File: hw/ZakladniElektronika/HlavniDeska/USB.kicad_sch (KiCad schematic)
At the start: 18 parts, among them J2 USB_C_Receptacle_USB2.0, U13 TPD4E02B04DQA, U4 AP33772

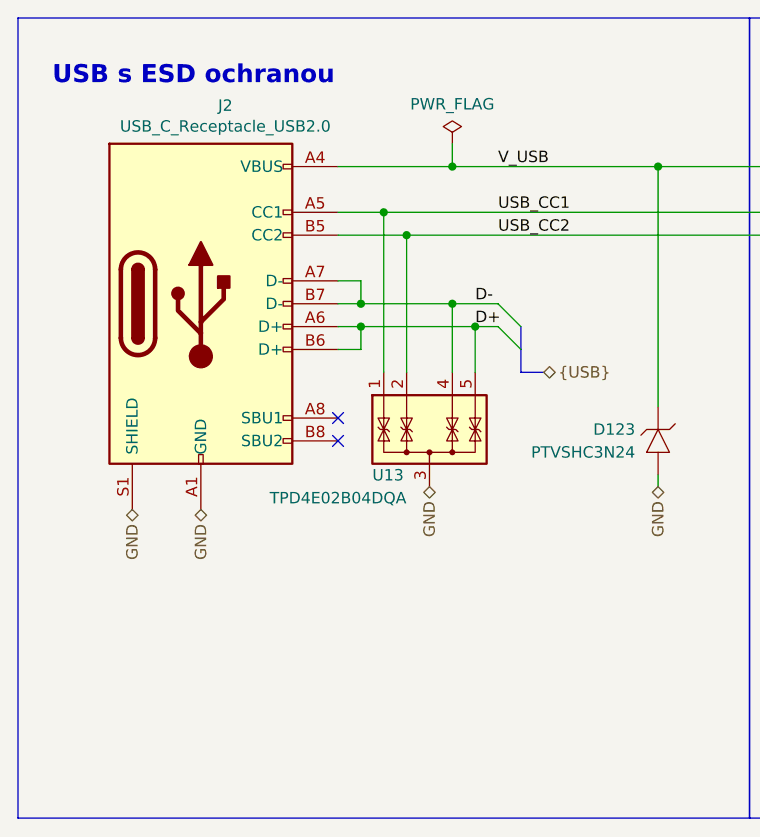
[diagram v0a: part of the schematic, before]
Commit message: WIP
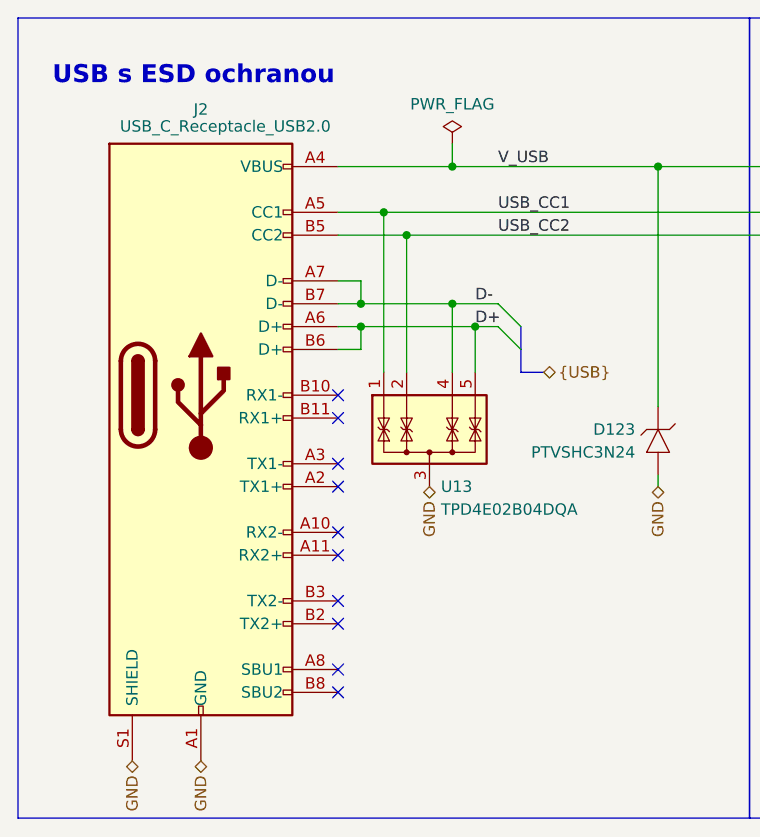
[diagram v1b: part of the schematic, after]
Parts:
- J2: symbol Connector:USB_C_Receptacle_USB2.0 -> Connector:USB_C_Receptacle
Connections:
- no-connect marks 7 -> 15
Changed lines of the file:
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@@
   )
   (no_connect (at 220.98 100.33))
+  (no_connect (at 86.36 107.95))
   (no_connect (at 220.98 110.49))
+  (no_connect (at 86.36 123.19))
+  (no_connect (at 86.36 100.33))
+  (no_connect (at 86.36 115.57))
+  (no_connect (at 86.36 125.73))
+  (no_connect (at 86.36 102.87))
   (no_connect (at 86.36 95.25))
-  (no_connect (at 86.36 97.79))
+  (no_connect (at 86.36 92.71))
+  (no_connect (at 86.36 110.49))
+  (no_connect (at 86.36 118.11))
   (no_connect (at 220.98 81.28))
   (no_connect (at 220.98 90.17))
@@
     (effects (font (size 1.27 1.27)) (justify right))
   )
-  (hierarchical_label "GND" (shape bidirectional) (at 71.12 105.41 270) (fields_autoplaced)
-    (effects (font (size 1.27 1.27)) (justify right))
-  )
-  (hierarchical_label "GND" (shape bidirectional) (at 63.5 105.41 270) (fields_autoplaced)
+  (hierarchical_label "GND" (shape bidirectional) (at 71.12 133.35 270) (fields_autoplaced)
+    (effects (font (size 1.27 1.27)) (justify right))
+  )
+  (hierarchical_label "GND" (shape bidirectional) (at 63.5 133.35 270) (fields_autoplaced)
     (effects (font (size 1.27 1.27)) (justify right))
   )
@@
     )
   )
-  (symbol (lib_id "Connector:USB_C_Receptacle_USB2.0") (at 71.12 82.55 0) (unit 1)
-    (in_bom yes) (on_board yes) (dnp no)
-    (property "Reference" "J2" (at 73.8378 60.5282 0)
+  (symbol (lib_id "Connector:USB_C_Receptacle") (at 71.12 92.71 0) (unit 1)
+    (in_bom yes) (on_board yes) (dnp no)
+    (property "Reference" "J2" (at 71.12 60.96 0)
       (effects (font (size 1.27 1.27)))
     )
@@
       (effects (font (size 1.27 1.27)))
     )
-    (property "Footprint" "RKL-Connectors:USB31-TYPEC-33141-2FS" (at 74.93 82.55 0)
-      (effects (font (size 1.27 1.27)) hide)
-    )
-    (property "Datasheet" "https://www.usb.org/sites/default/files/documents/usb_type-c.zip" (at 74.93 82.55 0)
-      (effects (font (size 1.27 1.27)) hide)
-    )
-    (property "LCSC" "C480368" (at 71.12 82.55 0)
-      (effects (font (size 1.27 1.27)) hide)
-    )
-    (property "JLCPCB_CORRECTION" "0;-1;0" (at 71.12 82.55 0)
-      (effects (font (size 1.27 1.27)) hide)
-    )
-    (property "Basic/Extended" "E" (at 71.12 82.55 0)
+    (property "Footprint" "RKL-Connectors:USB31-TYPEC-33141-2FS" (at 74.93 92.71 0)
+      (effects (font (size 1.27 1.27)) hide)
+    )
+    (property "Datasheet" "https://www.usb.org/sites/default/files/documents/usb_type-c.zip" (at 74.93 92.71 0)
+      (effects (font (size 1.27 1.27)) hide)
+    )
+    (property "LCSC" "C480368" (at 71.12 63.5 0)
+      (effects (font (size 1.27 1.27)) hide)
+    )
+    (property "JLCPCB_CORRECTION" "0;-1;0" (at 71.12 58.42 0)
+      (effects (font (size 1.27 1.27)) hide)
+    )
+    (property "Basic/Extended" "E" (at 71.12 60.96 0)
       (effects (font (size 1.27 1.27)) hide)
     )
     (pin "A1")
+    (pin "A10")
+    (pin "A11")
     (pin "A12")
+    (pin "A2")
+    (pin "A3")
     (pin "A4")
     (pin "A5")
@@
     (pin "A9")
     (pin "B1")
+    (pin "B10")
+    (pin "B11")
     (pin "B12")
+    (pin "B2")
+    (pin "B3")
     (pin "B4")
     (pin "B5")
@@
   (symbol (lib_id "RKL-Uncategorized:TPD4E02B04DQA") (at 96.52 92.71 0) (unit 1)
     (in_bom yes) (on_board yes) (dnp no)
-    (property "Reference" "U13" (at 90.17 101.6 0)
-      (effects (font (size 1.27 1.27)) (justify left))
-    )
-    (property "Value" "TPD4E02B04DQA" (at 86.36 104.14 0)
-      (effects (font (size 1.27 1.27)))
+    (property "Reference" "U13" (at 97.79 102.87 0)
+      (effects (font (size 1.27 1.27)) (justify left))
+    )
+    (property "Value" "TPD4E02B04DQA" (at 97.79 105.41 0)
+      (effects (font (size 1.27 1.27)) (justify left))
     )
     (property "Footprint" "Package_SON:USON-10_2.5x1.0mm_P0.5mm" (at 96.52 92.71 0)
